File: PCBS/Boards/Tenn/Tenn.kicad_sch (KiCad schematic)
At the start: 34 parts, among them J1 Conn_01x02_Socket, J10 Conn_01x03_Male, J11 Conn_01x03_Male, J12 Conn_01x04_Female, J13 Conn_01x03_Male, J14 Conn_01x03_Male, J15 Conn_01x03_Male, J16 Conn_01x02_Male, J17 Conn_01x02_Male, J2 Conn_01x03_Male, J3 Conn_01x03_Male, J4 Conn_01x03_Male, J5 Conn_01x03_Male, J6 Conn_01x03_Male, J7 Conn_01x03_Male, J8 Conn_01x03_Male, J9 Conn_01x03_Male, SW2 SW_Push, SW3 SW_Push, SW4 SW_SPDT, U1 L7805, U2 DRV8871DDA, U3 DRV8871DDA

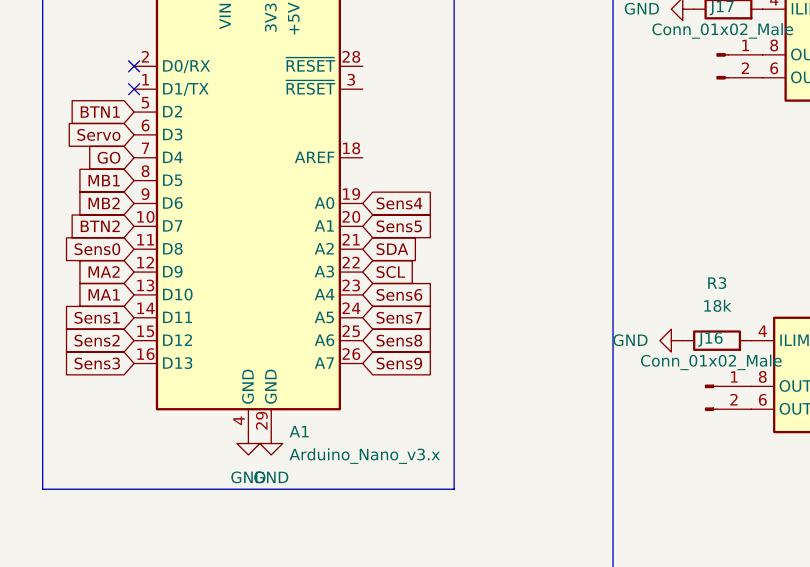
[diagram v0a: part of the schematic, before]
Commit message: updated README
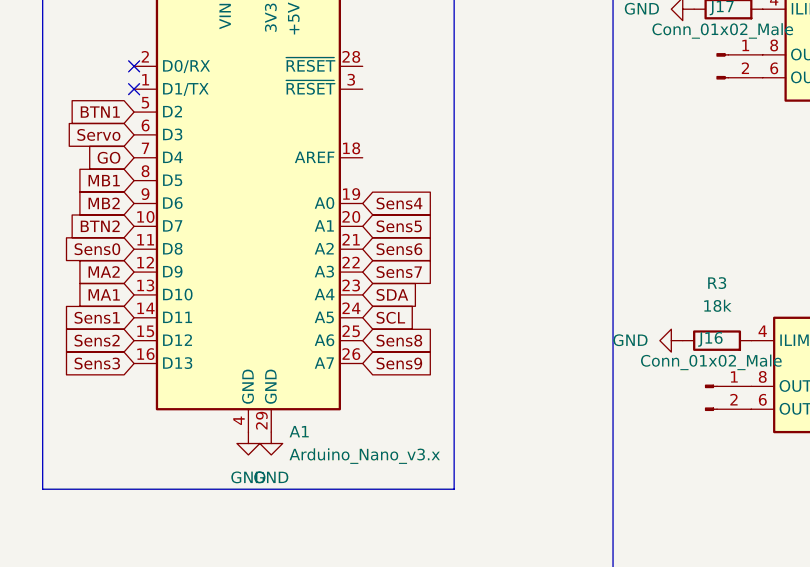
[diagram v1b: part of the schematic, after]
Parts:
- J12: footprint Connector_PinHeader_2.54mm:PinHeader_1x04_P2.54mm_Vertical -> Connector_PinSocket_2.54mm:PinSocket_1x04_P2.54mm_Vertical
- J16, J17: footprint Connector_PinSocket_2.54mm:PinSocket_1x02_P2.54mm_Vertical -> Connector_JST:JST_XH_B2B-XH-A_1x02_P2.50mm_Vertical
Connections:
- net SCL: now also A1.24 (A5); no longer A1.22 (A3)
- net SDA: now also A1.23 (A4); no longer A1.21 (A2)
- net Sens6: now also A1.21 (A2); no longer A1.23 (A4)
- net Sens7: now also A1.22 (A3); no longer A1.24 (A5)
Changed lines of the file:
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@@
     )
   )
-  (global_label "SDA" (shape input) (at 175.26 115.57 0) (fields_autoplaced)
+  (global_label "SDA" (shape input) (at 175.26 120.65 0) (fields_autoplaced)
     (effects (font (size 1.27 1.27)) (justify left))
-    (property "Intersheetrefs" "${INTERSHEET_REFS}" (at 181.2412 115.4906 0)
+    (property "Intersheetrefs" "${INTERSHEET_REFS}" (at 181.2412 120.5706 0)
       (effects (font (size 1.27 1.27)) (justify left) hide)
     )
@@
     )
   )
-  (global_label "Sens6" (shape input) (at 175.26 120.65 0) (fields_autoplaced)
+  (global_label "Sens6" (shape input) (at 175.26 115.57 0) (fields_autoplaced)
     (effects (font (size 1.27 1.27)) (justify left))
-    (property "Intersheetrefs" "${INTERSHEET_REFS}" (at 183.3579 120.5706 0)
+    (property "Intersheetrefs" "${INTERSHEET_REFS}" (at 183.3579 115.4906 0)
       (effects (font (size 1.27 1.27)) (justify left) hide)
     )
@@
     )
   )
-  (global_label "SCL" (shape input) (at 175.26 118.11 0) (fields_autoplaced)
+  (global_label "SCL" (shape input) (at 175.26 123.19 0) (fields_autoplaced)
     (effects (font (size 1.27 1.27)) (justify left))
-    (property "Intersheetrefs" "${INTERSHEET_REFS}" (at 181.1807 118.0306 0)
+    (property "Intersheetrefs" "${INTERSHEET_REFS}" (at 181.1807 123.1106 0)
       (effects (font (size 1.27 1.27)) (justify left) hide)
     )
   )
-  (global_label "Sens7" (shape input) (at 175.26 123.19 0) (fields_autoplaced)
+  (global_label "Sens7" (shape input) (at 175.26 118.11 0) (fields_autoplaced)
     (effects (font (size 1.27 1.27)) (justify left))
-    (property "Intersheetrefs" "${INTERSHEET_REFS}" (at 183.3579 123.1106 0)
+    (property "Intersheetrefs" "${INTERSHEET_REFS}" (at 183.3579 118.0306 0)
       (effects (font (size 1.27 1.27)) (justify left) hide)
     )
@@
       (effects (font (size 1.27 1.27)))
     )
-    (property "Footprint" "Connector_PinSocket_2.54mm:PinSocket_1x02_P2.54mm_Vertical" (at 213.36 130.81 0)
+    (property "Footprint" "Connector_JST:JST_XH_B2B-XH-A_1x02_P2.50mm_Vertical" (at 213.36 130.81 0)
       (effects (font (size 1.27 1.27)) hide)
     )
@@
       (effects (font (size 1.27 1.27)))
     )
-    (property "Footprint" "Connector_PinSocket_2.54mm:PinSocket_1x02_P2.54mm_Vertical" (at 214.63 93.98 0)
+    (property "Footprint" "Connector_JST:JST_XH_B2B-XH-A_1x02_P2.50mm_Vertical" (at 214.63 93.98 0)
       (effects (font (size 1.27 1.27)) hide)
     )
@@
       (effects (font (size 1.27 1.27)))
     )
-    (property "Footprint" "Connector_PinHeader_2.54mm:PinHeader_1x04_P2.54mm_Vertical" (at 99.06 90.17 0)
-      (effects (font (size 1.27 1.27)) hide)
-    )
+    (property "Footprint" "Connector_PinSocket_2.54mm:PinSocket_1x04_P2.54mm_Vertical" (at 99.06 90.17 0)
+      (effects (font (size 1.27 1.27)) hide)
+    )
